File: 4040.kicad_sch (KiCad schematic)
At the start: 127 parts, among them J1 USB_C_Receptacle_USB2.0_16P, SW1 SW_Push, U2 ATmega32U4-A, Y1 16MHz

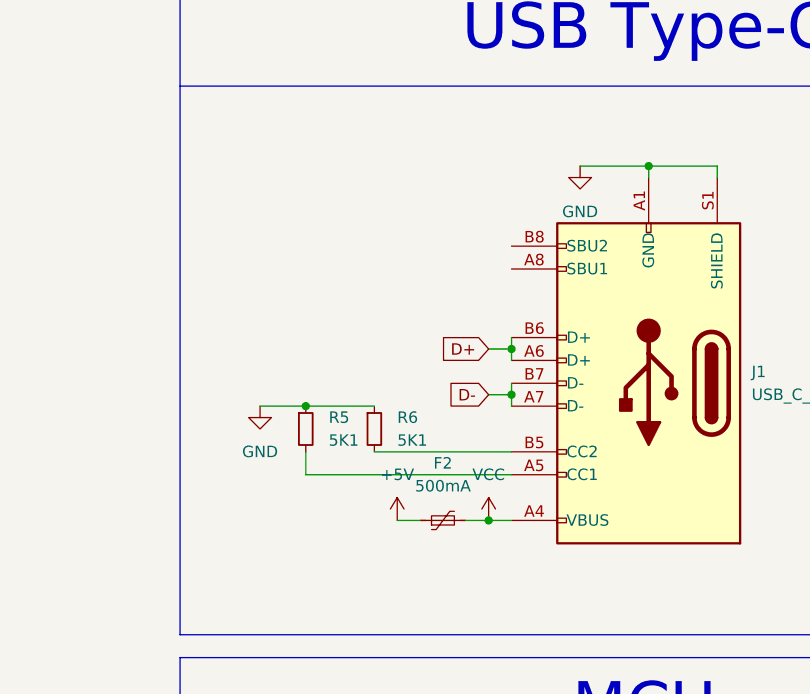
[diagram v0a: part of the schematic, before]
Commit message: main
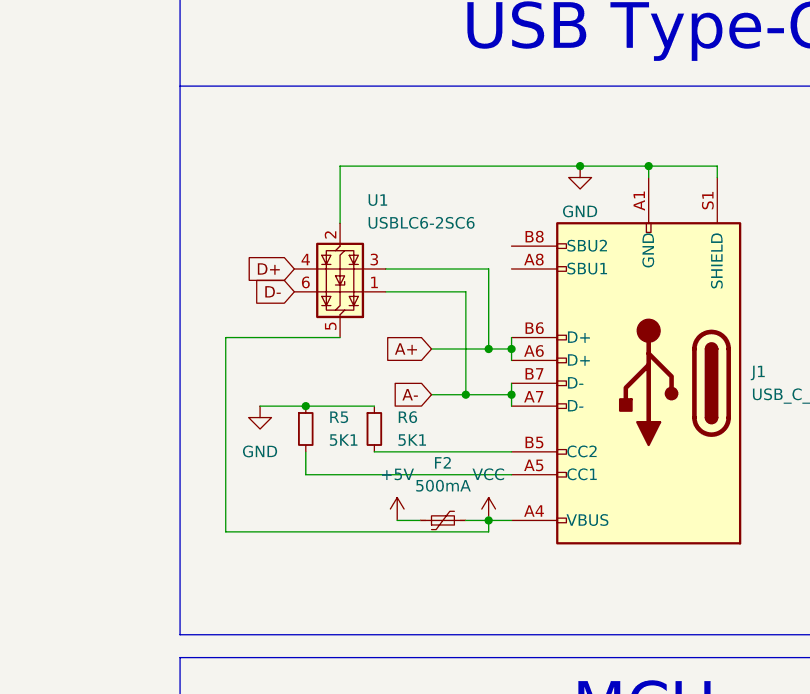
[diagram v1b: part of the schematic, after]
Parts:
- added U1: USBLC6-2SC6, Package_TO_SOT_SMD:SOT-23-6, symbol Power_Protection:USBLC6-2SC6
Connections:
- net D+: now also U1.4 (I/O2); no longer J1.A6 (D+), J1.B6 (D+)
- net D-: now also U1.6 (I/O1); no longer J1.A7 (D-), J1.B7 (D-)
- net GND: now also U1.2 (GND)
- net VCC: now also U1.5 (VBUS)
- new net A+: J1.A6 (D+), J1.B6 (D+), U1.3 (I/O2)
- new net A-: J1.A7 (D-), J1.B7 (D-), U1.1 (I/O1)
